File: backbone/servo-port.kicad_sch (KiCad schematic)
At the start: 41 parts, among them J1201 RS-485 JST EH 4p, J1202 TTL JST EH 3p, U1201 SP3485EN-L/TR, U1202 SN74LVC2G241DCU, U1203 TPS16630PWPR, U1204 TPS25961DRVR

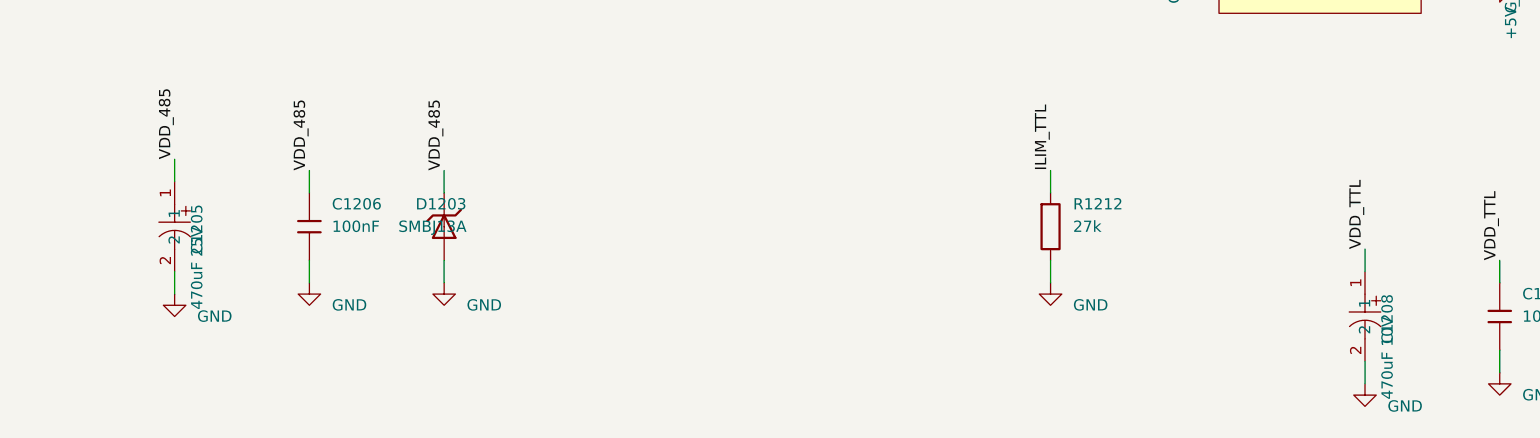
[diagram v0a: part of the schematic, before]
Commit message: schematics
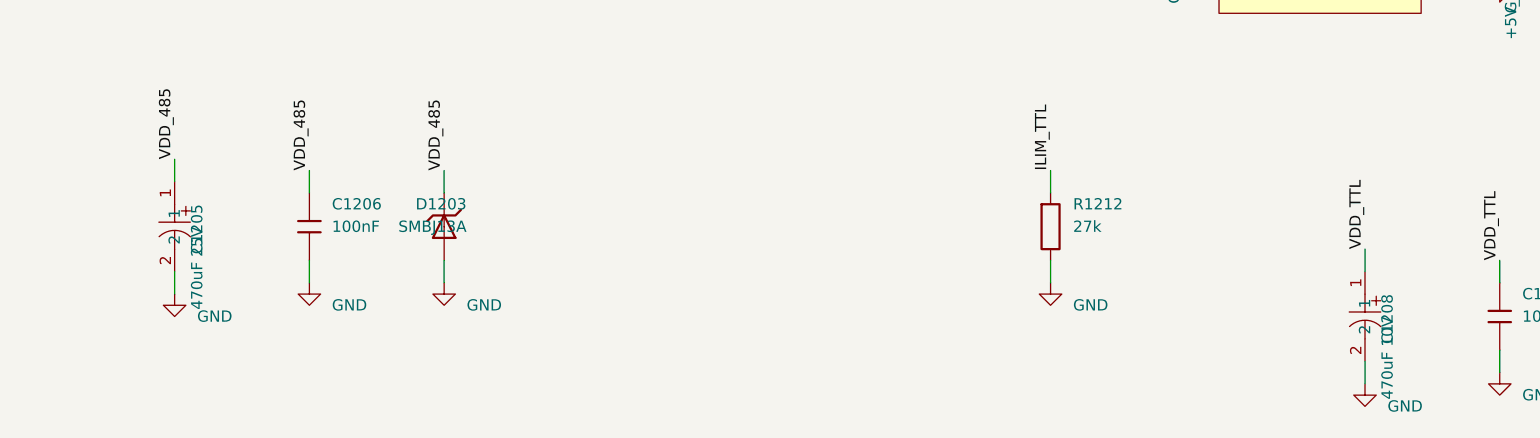
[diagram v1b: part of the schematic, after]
